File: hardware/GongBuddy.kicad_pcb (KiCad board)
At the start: 2 copper layers, 39.2 x 59.5 mm, 49 parts, among them J1 10103594-0001LF, J2 Conn_ARM_JTAG_SWD_10, J3 2908-05WB-MG, J4 Conn_01x10, J5 Conn_01x02, J7 Conn_Coaxial, U1 TPS7A19, U2 USBLC6-2SC6, U3 MCP73831T-2ACI_OT, U4 ST_Sensortile, U5 RFM95W-915S2, U6 MCP23S08

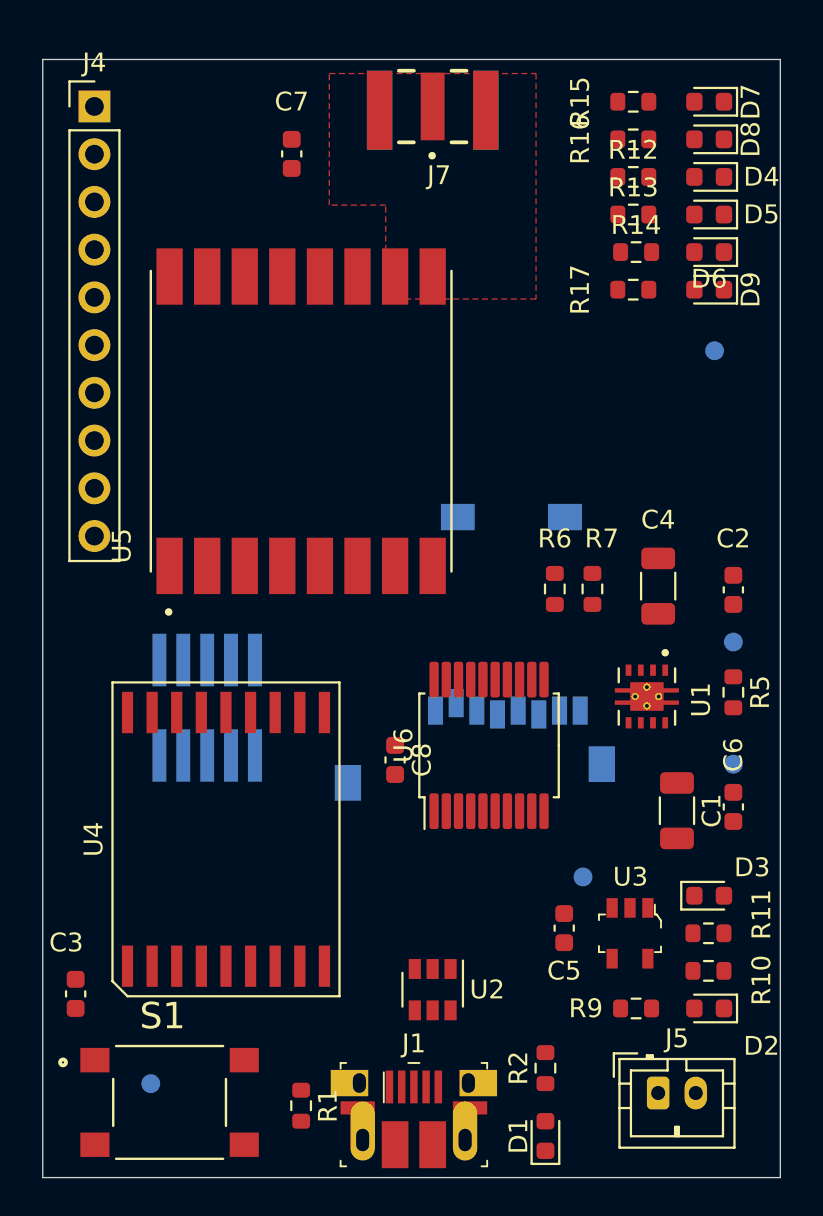
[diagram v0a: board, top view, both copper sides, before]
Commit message: Added more files.
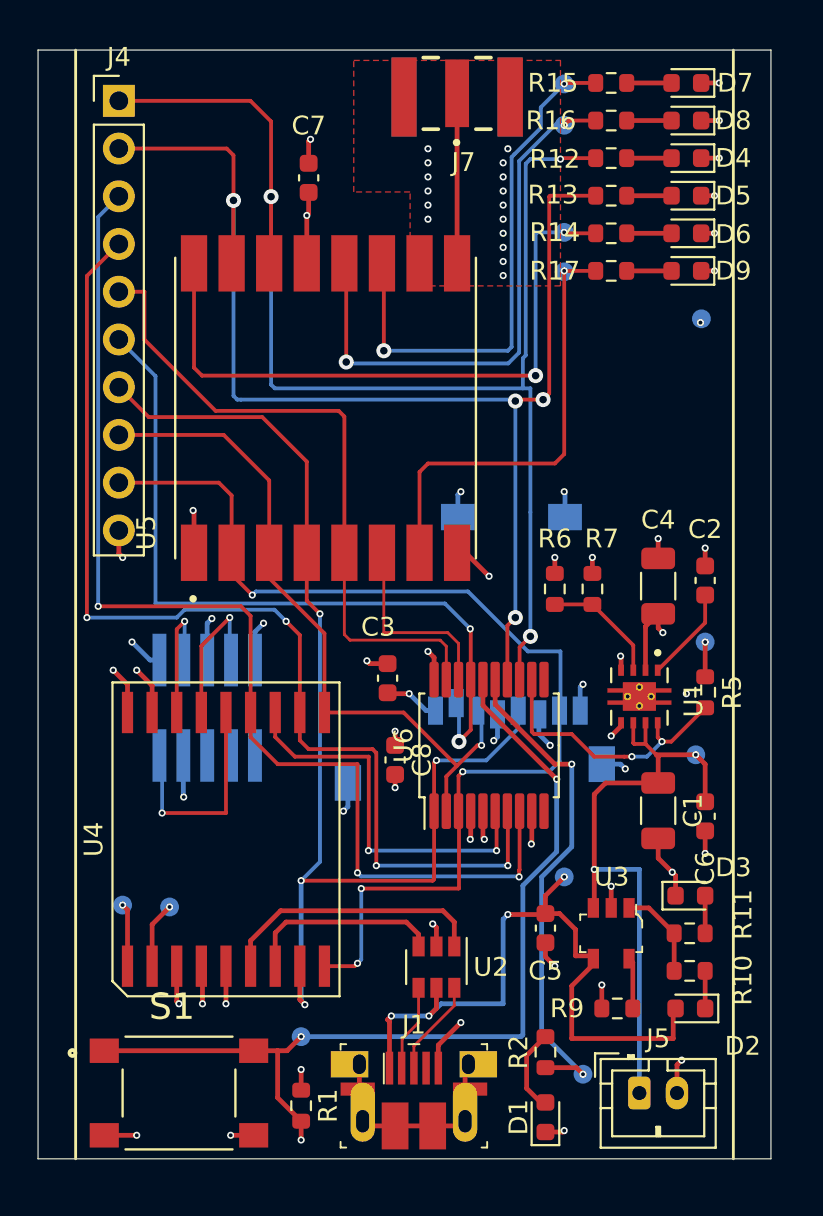
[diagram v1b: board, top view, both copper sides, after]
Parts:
- added TP10: TestPoint, TestPoint:TestPoint_Pad_D1.0mm, B.Cu at (66.0, 84.0)
- added TP11: TestPoint, TestPoint:TestPoint_Pad_D1.0mm, B.Cu at (67.0, 134.5)
- added TP12: TestPoint, TestPoint:TestPoint_Pad_D1.0mm, B.Cu at (66.0, 91.8)
- added TP6: TestPoint, TestPoint:TestPoint_Pad_D1.0mm, B.Cu at (42.5, 125.5)
- added TP7: TestPoint, TestPoint:TestPoint_Pad_D1.0mm, B.Cu at (52.0, 132.5)
- added TP8: TestPoint, TestPoint:TestPoint_Pad_D1.0mm, B.Cu at (66.0, 89.7)
- added TP9: TestPoint, TestPoint:TestPoint_Pad_D1.0mm, B.Cu at (66.0, 81.8)
- moved C3 23.6 mm to (56.6, 113.4)
- moved TP1 9.45 mm to (45.0, 125.6)
- moved TP4 2.06 mm to (73.0, 117.5)
- moved TP5 1.84 mm to (73.3, 94.3)
- moved R14 1.66 mm to (68.5, 89.8)
- moved C2 1.58 mm to (73.5, 108.2)
- moved C6 1.58 mm to (73.5, 120.8), turned to 270 degrees
- moved D4 1.57 mm to (72.5, 85.8)
- moved D5 1.57 mm to (72.5, 87.8)
- moved D6 1.57 mm to (72.5, 89.8)
- moved D7 1.57 mm to (72.5, 81.8)
- moved D8 1.57 mm to (72.5, 83.8)
- moved D9 1.57 mm to (72.5, 91.8)
- moved C7 1.56 mm to (52.4, 86.8)
- moved R12 1.54 mm to (68.5, 85.8)
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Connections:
- J4 pad 7: /SPI_MOSI -> /SPI_CLK
- J4 pad 8: /SPI_CLK -> /SPI_MOSI
- U1 pad 10: (no net) -> GND
- U1 pad 11: (no net) -> GND
- U1 pad 12: (no net) -> GND
- U1 pad 13: (no net) -> GND
- U6 pad 12: /DIO0 -> /PG
- U6 pad 13: /DIO1 -> /DIO0
- U6 pad 14: /LED1 -> /DIO1
- U6 pad 15: /BUTTON1 -> /LED1
- U6 pad 16: /LORA_CS -> /BUTTON1
- U6 pad 17: /LORA_RESET -> /SD_CS
- U6 pad 18: /PG -> /LORA_RESET
- U6 pad 19: /SD_CS -> /LORA_CS
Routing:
- net /DIO0: track 0.00 -> 71.8 mm, vias 0 -> 3
- net /DIO1: track 0.00 -> 68.0 mm, vias 0 -> 4
- net GND: track 0.00 -> 67.1 mm, vias 0 -> 61
- net /SPI_CLK: track 0.00 -> 63.1 mm, vias 0 -> 4
- net /IO_INT: track 0.00 -> 61.3 mm, vias 0 -> 3
- net /IO_CS: track 0.00 -> 58.5 mm, vias 0 -> 4
- net /SPI_MISO: track 0.00 -> 58.5 mm, vias 0 -> 4
- net /BUTTON1: track 0.00 -> 49.2 mm, vias 0 -> 3
- net /SD_CS: track 0.00 -> 40.5 mm, vias 0 -> 2
- net /SPI_MOSI: track 0.00 -> 37.2 mm, vias 0 -> 1
- net VBUS: track 0.00 -> 36.2 mm, vias 0 -> 4
- net /LORA_CS: track 0.00 -> 35.3 mm
- net /DIO2: track 0.00 -> 34.8 mm, vias 0 -> 2
- net /VBAT: track 0.00 -> 34.3 mm, vias 0 -> 2
- net /DIO4: track 0.00 -> 30.0 mm, vias 0 -> 2
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- added copper zone on In2.Cu, net GND
- added copper zone on In1.Cu, net VCC
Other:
- board size 39.2 x 59.5 mm -> 39 x 59 mm
- copper layers 2 -> 4
- net class Default: clearance 0.2 -> 0.127; trace_width 0.25 -> 0.1524; via_dia 0.8 -> 0.381; via_drill 0.4 -> 0.2032
- rule trace_clearance: 0.2 -> 0.127
- rule trace_min: 0.2 -> 0.1016
- rule via_min_drill: 0.3 -> 0.2032
- rule via_min_size: 0.4 -> 0.381
- board text added: "GongBuddy Rev B Copyright 2021 Nick Butts"
- board text removed: "GongBuddy Rev A Copyright 2020 Nick Butts"
